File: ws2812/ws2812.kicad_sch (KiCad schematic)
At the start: 8 parts, among them J1 STM32WORLD_BOARD, J2 STM32WORLD_CONNECTOR_1, J3 STM32WORLD_CONNECTOR_2, U1 WS2812E, U2 WS2812E, U3 WS2812E, U4 WS2812E, U5 WS2812E

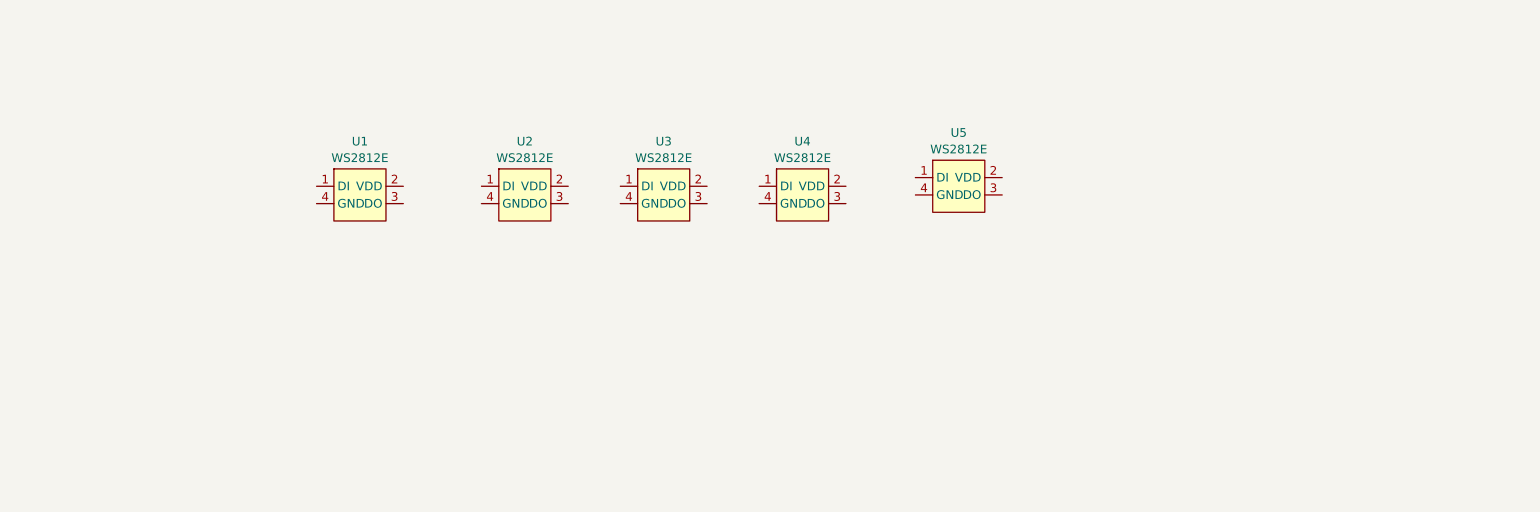
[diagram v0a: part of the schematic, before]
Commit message: Hmmmm
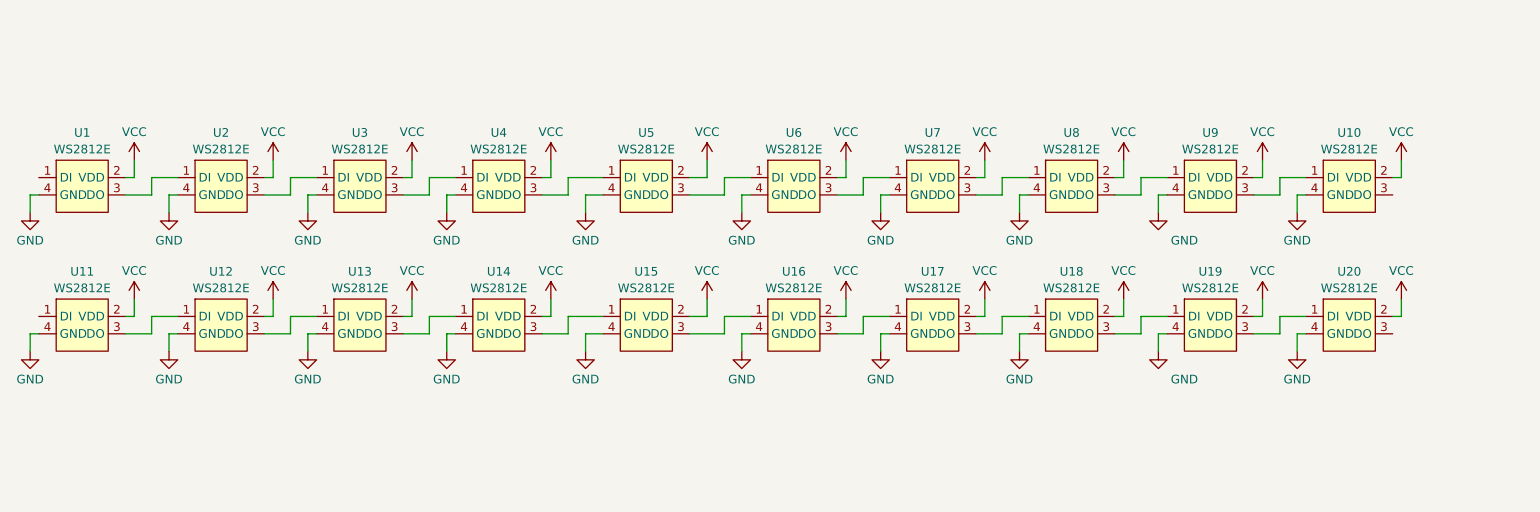
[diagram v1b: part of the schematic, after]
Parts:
- added U10, U11, U12, U13, U14, U15, U16, U17, U18, U19, U20, U6, U7, U8, U9: WS2812E, stm32world:LED-SMD_4P-L3.7-W3.5-P1.75-BR-SK6812MINI, symbol stm32world:WS2812E-MINI-X1
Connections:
- net at U4.1 (DI): now also U3.3 (DO)
- net VCC: now reaches U4.2 (VDD)
- net VCC: now also U1.2 (VDD), U2.2 (VDD), U3.2 (VDD), U5.2 (VDD), U10.2 (VDD), U11.2 (VDD), U12.2 (VDD), U13.2 (VDD), U14.2 (VDD), U15.2 (VDD), U16.2 (VDD), U17.2 (VDD), U18.2 (VDD), U19.2 (VDD), U20.2 (VDD), U6.2 (VDD), U7.2 (VDD), U8.2 (VDD), U9.2 (VDD)
- net at U4.3 (DO): now also U5.1 (DI)
- net GND: now reaches U4.4 (GND)
- net GND: now also U1.4 (GND), U2.4 (GND), U3.4 (GND), U5.4 (GND), U10.4 (GND), U11.4 (GND), U12.4 (GND), U13.4 (GND), U14.4 (GND), U15.4 (GND), U16.4 (GND), U17.4 (GND), U18.4 (GND), U19.4 (GND), U20.4 (GND), U6.4 (GND), U7.4 (GND), U8.4 (GND), U9.4 (GND)
- net at U2.1 (DI): now also U1.3 (DO)
- net at U2.3 (DO): now also U3.1 (DI)
- net at U5.3 (DO): now also U6.1 (DI)
- new net: U6.3 (DO), U7.1 (DI)
- new net: U7.3 (DO), U8.1 (DI)
- new net: U12.3 (DO), U13.1 (DI)
- new net: U13.3 (DO), U14.1 (DI)
- new net: U15.3 (DO), U16.1 (DI)
- new net: U16.3 (DO), U17.1 (DI)
- new net: U8.3 (DO), U9.1 (DI)
- new net: U19.3 (DO), U20.1 (DI)
- new net: U14.3 (DO), U15.1 (DI)
- new net: U17.3 (DO), U18.1 (DI)
- new net: U18.3 (DO), U19.1 (DI)
- new net: U11.3 (DO), U12.1 (DI)
- new net: U10.1 (DI), U9.3 (DO)
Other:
- moved on the sheet: U1, U2, U3, U4, U5
